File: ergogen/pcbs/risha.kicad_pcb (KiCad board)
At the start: 2 copper layers, 100 x 81 mm, 23 parts

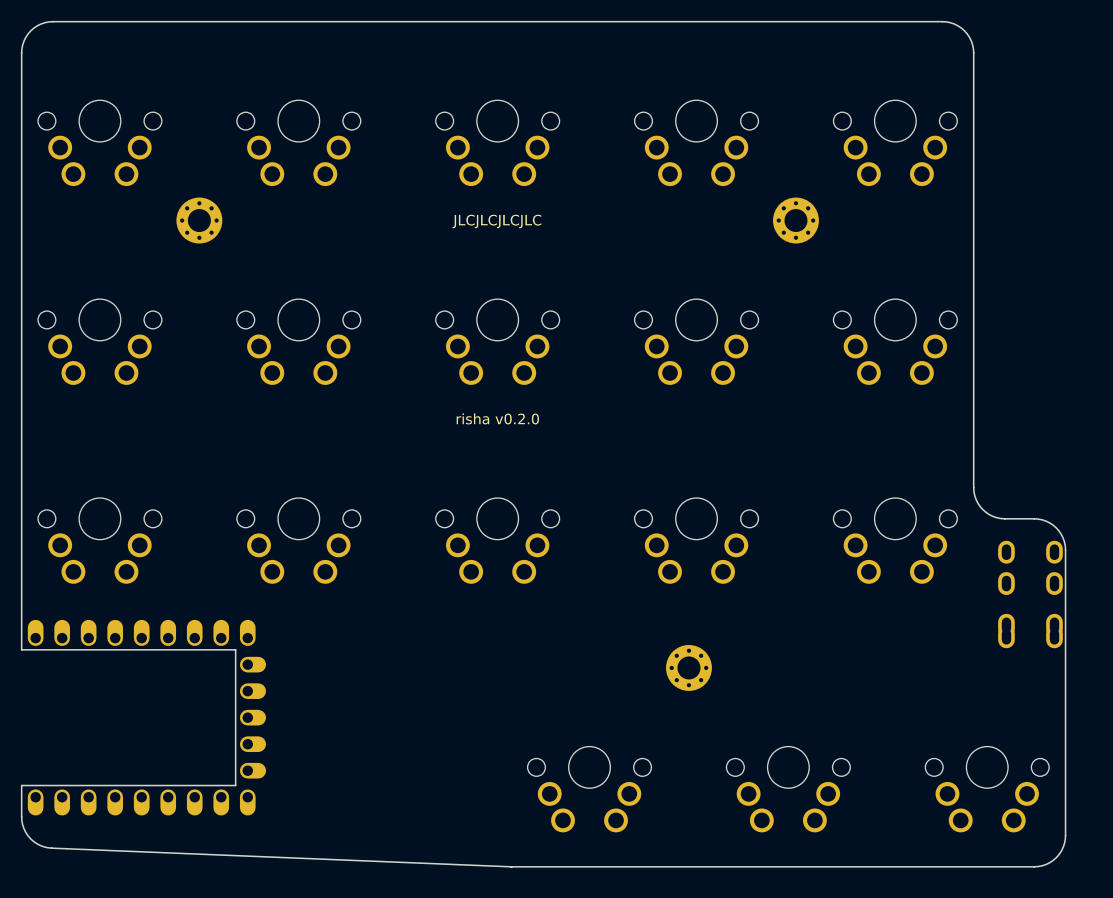
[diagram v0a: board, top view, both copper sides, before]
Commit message: v0.3.0 (#3)
* v0.3.0 prototypes ordered
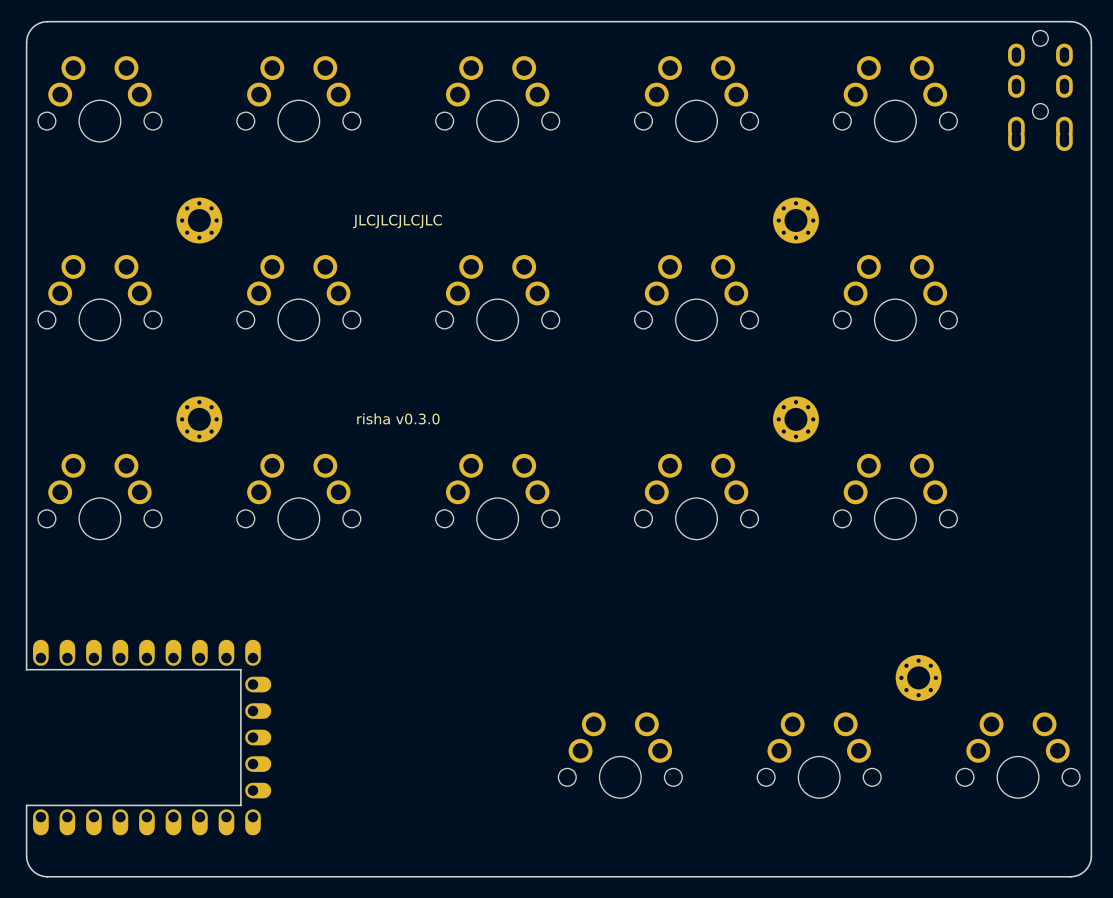
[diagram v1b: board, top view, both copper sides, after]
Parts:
- added _7: , MountingHole_2.2mm_M2_Pad_Via, F.Cu at (219.1, 123.8)
- added _8: , MountingHole_2.2mm_M2_Pad_Via, F.Cu at (230.8, 167.6)
- moved _4 52.6 mm to (161.9, 142.9)
- moved TRRS1 47.6 mm to (244.8, 104.8)
- moved _6 19.1 mm to (219.1, 142.9)
- moved S16 3.10 mm to (202.2, 177.2), turned to 0 degrees
- moved S17 3.10 mm to (221.3, 177.2), turned to 0 degrees
- moved S18 3.10 mm to (240.3, 177.2), turned to 0 degrees
- moved ? 1.97 mm to (156.9, 173.4)
- turned S1 to 0 degrees
- turned S10 to 0 degrees
- turned S11 to 0 degrees
- turned S12 to 0 degrees
- turned S13 to 0 degrees
- turned S14 to 0 degrees
- turned S15 to 0 degrees
- turned S2 to 0 degrees
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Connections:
- ? pad 14: matrix_inner_top -> matrix_inner_bottom
- ? pad 16: matrix_inner_bottom -> matrix_inner_top
- ? pad 17: thumbfan_near_home -> thumbfan_far_home
- ? pad 19: thumbfan_far_home -> thumbfan_near_home
- ? pad 4: matrix_ring_top -> matrix_ring_bottom
- ? pad 6: matrix_ring_bottom -> matrix_ring_top
- ? pad 7: matrix_middle_top -> matrix_middle_bottom
- ? pad 9: matrix_middle_bottom -> matrix_middle_top
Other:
- board size 100 x 81 mm -> 102 x 81.9 mm
- board text added: "risha v0.3.0"
- board text removed: "risha v0.2.0"
